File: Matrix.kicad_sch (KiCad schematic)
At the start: 140 parts, among them SW3 RotaryEncoder_Switch

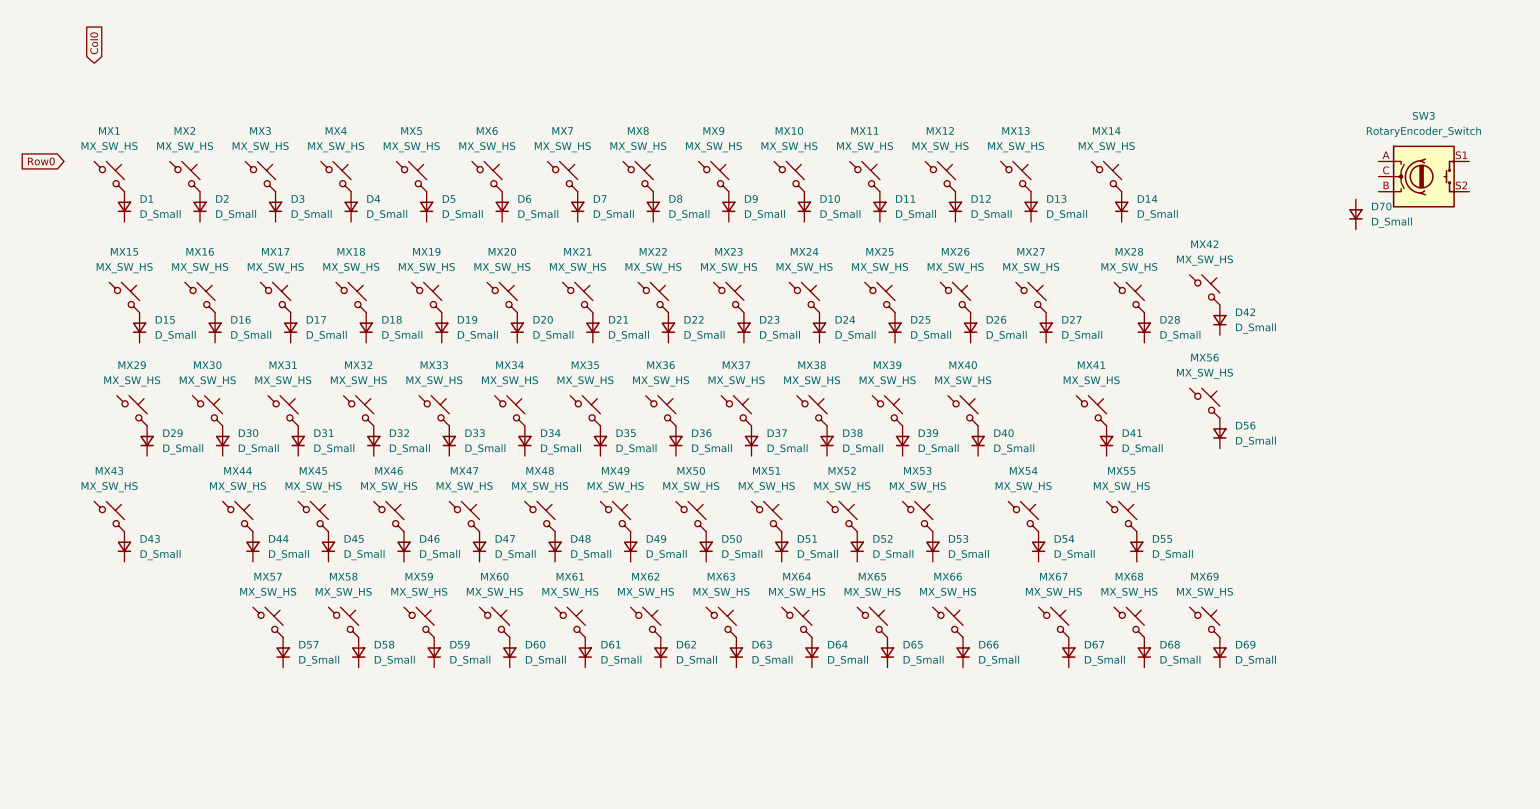
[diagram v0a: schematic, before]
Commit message: Finished switch matrix
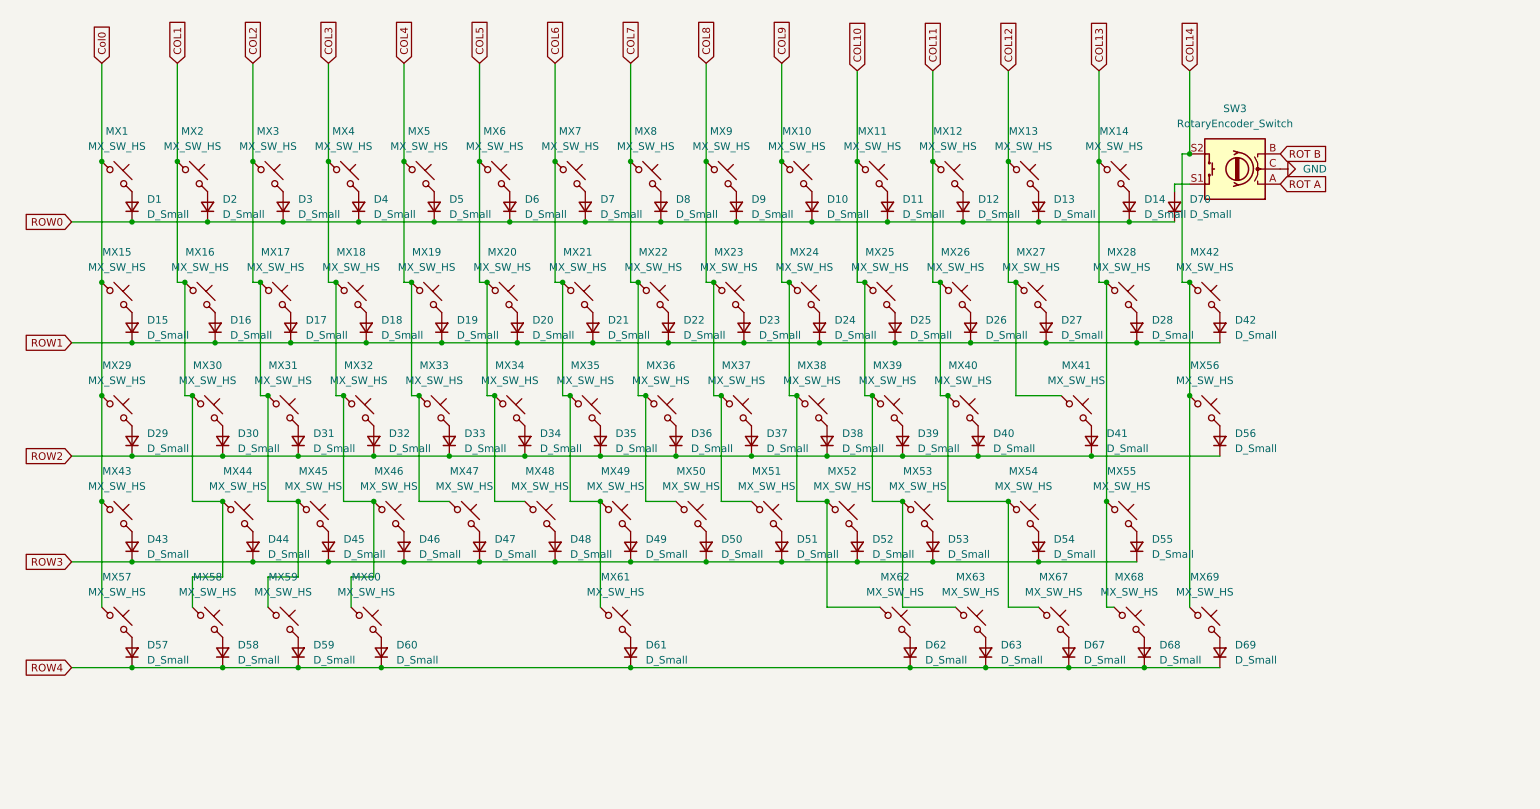
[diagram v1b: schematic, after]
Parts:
- removed D64, D65, D66: D_Small, symbol Device:D_Small
- removed MX64, MX65, MX66: MX_SW_HS, PCM_marbastlib-mx:SW_MX_HS_1u, symbol PCM_marbastlib-mx:MX_SW_HS
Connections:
- net Col0: now also MX1.1, MX15.1, MX29.1, MX43.1, MX57.1
- net COL9: now reaches MX38.1
- net COL9: now also MX10.1, MX24.1, MX52.1, MX62.1
- net COL1: now reaches MX2.1
- net COL1: now also MX16.1, MX30.1, MX44.1, MX58.1
- net COL8: now reaches MX23.1
- net COL8: now also MX37.1, MX51.1, MX9.1
- net COL3: now reaches MX32.1
- net COL3: now also MX18.1, MX4.1, MX46.1, MX60.1
- net COL12: now reaches MX41.1
- net COL12: now also MX13.1, MX27.1
- net COL7: now reaches MX50.1
- net COL7: now also MX22.1, MX36.1, MX8.1
- net COL6: now reaches MX21.1
- net COL6: now also MX35.1, MX49.1, MX61.1, MX7.1
- net ROW2: now reaches D38.1 (K)
- net ROW2: now also D29.1 (K), D30.1 (K), D31.1 (K), D32.1 (K), D33.1 (K), D34.1 (K), D35.1 (K), D36.1 (K), D37.1 (K), D39.1 (K), D40.1 (K), D41.1 (K), D56.1 (K)
- net ROW0: now reaches D70.1 (K)
- net ROW0: now also D1.1 (K), D10.1 (K), D11.1 (K), D12.1 (K), D13.1 (K), D14.1 (K), D2.1 (K), D3.1 (K), D4.1 (K), D5.1 (K), D6.1 (K), D7.1 (K), D8.1 (K), D9.1 (K)
- net at D70.2 (A): now also SW3.S1
- net ROW4: now reaches D62.1 (K)
- net ROW4: now also D57.1 (K), D58.1 (K), D59.1 (K), D60.1 (K), D61.1 (K), D63.1 (K), D67.1 (K), D68.1 (K), D69.1 (K)
- net ROW1: now reaches D23.1 (K)
- net ROW1: now also D15.1 (K), D16.1 (K), D17.1 (K), D18.1 (K), D19.1 (K), D20.1 (K), D21.1 (K), D22.1 (K), D24.1 (K), D25.1 (K), D26.1 (K), D27.1 (K), D28.1 (K), D42.1 (K)
- net COL11: now reaches MX40.1
- net COL11: now also MX12.1, MX26.1, MX54.1, MX67.1
- net COL4: now reaches MX5.1
- net COL4: now also MX19.1, MX33.1, MX47.1
- net ROW3: now reaches D49.1 (K)
- net ROW3: now also D43.1 (K), D44.1 (K), D45.1 (K), D46.1 (K), D47.1 (K), D48.1 (K), D50.1 (K), D51.1 (K), D52.1 (K), D53.1 (K), D54.1 (K), D55.1 (K)
- net COL5: now reaches MX34.1
- net COL5: now also MX20.1, MX48.1, MX6.1
- net COL13: now reaches MX55.1
- net COL13: now also MX14.1, MX28.1, MX68.1
- net COL14: now reaches MX56.1
- net COL14: now also MX42.1, MX69.1, SW3.S2
- net COL2: now reaches MX59.1
- net COL2: now also MX17.1, MX3.1, MX31.1, MX45.1
- net COL10: now reaches MX39.1
- net COL10: now also MX11.1, MX25.1, MX53.1, MX63.1
- net ROT A: now reaches SW3.A
- net ROT B: now reaches SW3.B
- net GND: now reaches SW3.C
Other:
- moved on the sheet: D1, D10, D11, D12, D13, D14, D15, D2, D28, D29, D3, D4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

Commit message: idk
dont remember what i changed lol i think it should be led shit
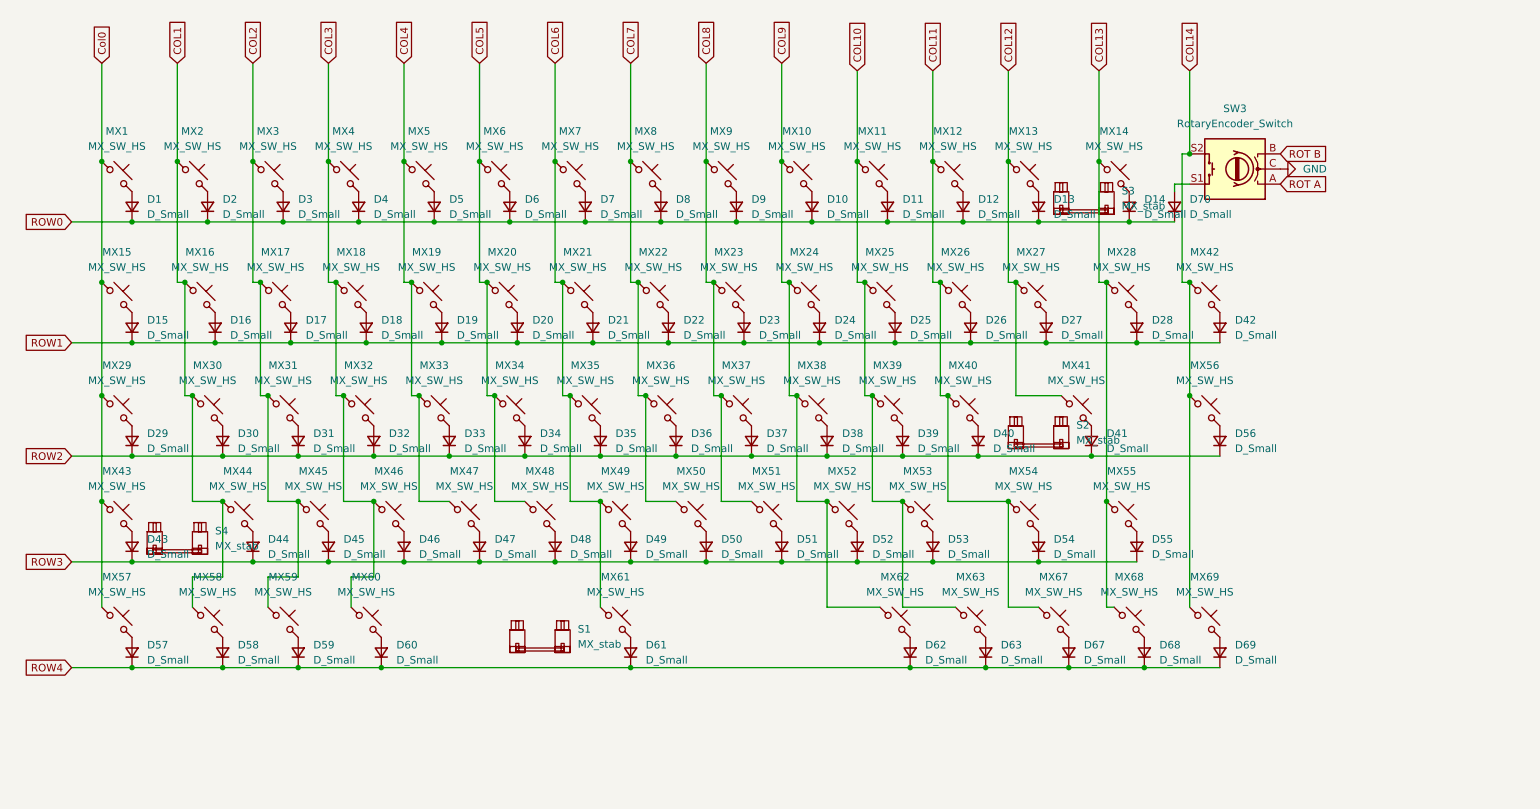
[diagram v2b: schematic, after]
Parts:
- added S1, S2, S3, S4: MX_stab, PCM_marbastlib-mx:STAB_MX_P_6.25u, symbol PCM_marbastlib-mx:MX_stab
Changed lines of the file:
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@@
+    )
+  )
+  (symbol (lib_id "PCM_marbastlib-mx:MX_stab") (at 191.77 55.88 0) (unit 1)
+    (in_bom yes) (on_board yes) (dnp no) (fields_autoplaced)
+    (property "Reference" "S3" (at 198.12 54.483 0)
+      (effects (font (size 1.27 1.27)) (justify left))
+    )
+    (property "Value" "MX_stab" (at 198.12 57.023 0)
+      (effects (font (size 1.27 1.27)) (justify left))
+    )
+    (property "Footprint" "PCM_marbastlib-mx:STAB_MX_P_6.25u" (at 191.77 55.88 0)
+      (effects (font (size 1.27 1.27)) hide)
+    )
+    (property "Datasheet" "" (at 191.77 55.88 0)
+      (effects (font (size 1.27 1.27)) hide)
+    )
+    (instances
+      (project "CODA65"
+        (path "/33ce4dbb-1d04-4b2d-9cde-6cc03c168fa4/fe44eb25-ace8-4884-b9d5-e7eefbf2b910"
+          (reference "S3") (unit 1)
+        )
+      )
     )
   )
@@
     )
   )
+  (symbol (lib_id "PCM_marbastlib-mx:MX_stab") (at 184.15 95.25 0) (unit 1)
+    (in_bom yes) (on_board yes) (dnp no) (fields_autoplaced)
+    (property "Reference" "S2" (at 190.5 93.853 0)
+      (effects (font (size 1.27 1.27)) (justify left))
+    )
+    (property "Value" "MX_stab" (at 190.5 96.393 0)
+      (effects (font (size 1.27 1.27)) (justify left))
+    )
+    (property "Footprint" "PCM_marbastlib-mx:STAB_MX_P_6.25u" (at 184.15 95.25 0)
+      (effects (font (size 1.27 1.27)) hide)
+    )
+    (property "Datasheet" "" (at 184.15 95.25 0)
+      (effects (font (size 1.27 1.27)) hide)
+    )
+    (instances
+      (project "CODA65"
+        (path "/33ce4dbb-1d04-4b2d-9cde-6cc03c168fa4/fe44eb25-ace8-4884-b9d5-e7eefbf2b910"
+          (reference "S2") (unit 1)
+        )
+      )
+    )
+  )
   (symbol (lib_id "PCM_marbastlib-mx:MX_SW_HS") (at 71.12 127 0) (unit 1)
     (in_bom yes) (on_board yes) (dnp no) (fields_autoplaced)
@@
     )
   )
+  (symbol (lib_id "PCM_marbastlib-mx:MX_stab") (at 39.37 113.03 0) (unit 1)
+    (in_bom yes) (on_board yes) (dnp no) (fields_autoplaced)
+    (property "Reference" "S4" (at 45.72 111.633 0)
+      (effects (font (size 1.27 1.27)) (justify left))
+    )
+    (property "Value" "MX_stab" (at 45.72 114.173 0)
+      (effects (font (size 1.27 1.27)) (justify left))
+    )
+    (property "Footprint" "PCM_marbastlib-mx:STAB_MX_P_6.25u" (at 39.37 113.03 0)
+      (effects (font (size 1.27 1.27)) hide)
+    )
+    (property "Datasheet" "" (at 39.37 113.03 0)
+      (effects (font (size 1.27 1.27)) hide)
+    )
+    (instances
+      (project "CODA65"
+        (path "/33ce4dbb-1d04-4b2d-9cde-6cc03c168fa4/fe44eb25-ace8-4884-b9d5-e7eefbf2b910"
+          (reference "S4") (unit 1)
+        )
+      )
+    )
+  )
   (symbol (lib_id "PCM_marbastlib-mx:MX_SW_HS") (at 120.65 91.44 0) (unit 1)
     (in_bom yes) (on_board yes) (dnp no) (fields_autoplaced)
@@
         )
       )
+    )
+  )
+  (symbol (lib_id "PCM_marbastlib-mx:MX_stab") (at 100.33 129.54 0) (unit 1)
+    (in_bom yes) (on_board yes) (dnp no) (fields_autoplaced)
+    (property "Reference" "S1" (at 106.68 128.143 0)
+      (effects (font (size 1.27 1.27)) (justify left))
+    )
+    (property "Value" "MX_stab" (at 106.68 130.683 0)
+      (effects (font (size 1.27 1.27)) (justify left))
+    )
+    (property "Footprint" "PCM_marbastlib-mx:STAB_MX_P_6.25u" (at 100.33 129.54 0)
+      (effects (font (size 1.27 1.27)) hide)
+    )
+    (property "Datasheet" "" (at 100.33 129.54 0)
+      (effects (font (size 1.27 1.27)) hide)
+    )
+    (instances
+      (project "CODA65"
+        (path "/33ce4dbb-1d04-4b2d-9cde-6cc03c168fa4/fe44eb25-ace8-4884-b9d5-e7eefbf2b910"
+          (reference "S1") (unit 1)
+        )
+      )

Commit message: assigned schema
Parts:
- D1, D10, D11, D12, D13, D14, D15, D16, D17, D18, D19, D2, D20, D21, D22, D23, D24, D25, D26, D27, D28, D29, D3, D30, D31, D32, D33, D34, D35, D36, D37, D38, D39, D4, D40, D41, D42, D43, D44, D45, D46, D47, D48, D49, D5, D50, D51, D52, D53, D54, D55, D56, D57, D58, D59, D6, D60, D61, D62, D63, D67, D68, D69, D7, D70, D8, D9: footprint (none) -> Diode_SMD:D_SOD-123
- MX15, MX28: footprint PCM_marbastlib-mx:SW_MX_HS_1u -> PCM_marbastlib-mx:SW_MX_HS_1.5u
- MX29, MX54: footprint PCM_marbastlib-mx:SW_MX_HS_1u -> PCM_marbastlib-mx:SW_MX_HS_1.75u
- MX58, MX63: footprint PCM_marbastlib-mx:SW_MX_HS_1u -> PCM_marbastlib-mx:SW_MX_HS_1.25u
- S2, S4: footprint PCM_marbastlib-mx:STAB_MX_P_6.25u -> PCM_marbastlib-mx:STAB_MX_P_2.25u
- S3: footprint PCM_marbastlib-mx:STAB_MX_P_6.25u -> PCM_marbastlib-mx:STAB_MX_P_2u
- SW3: footprint (none) -> Rotary_Encoder:RotaryEncoder_Alps_EC11E-Switch_Vertical_H20mm

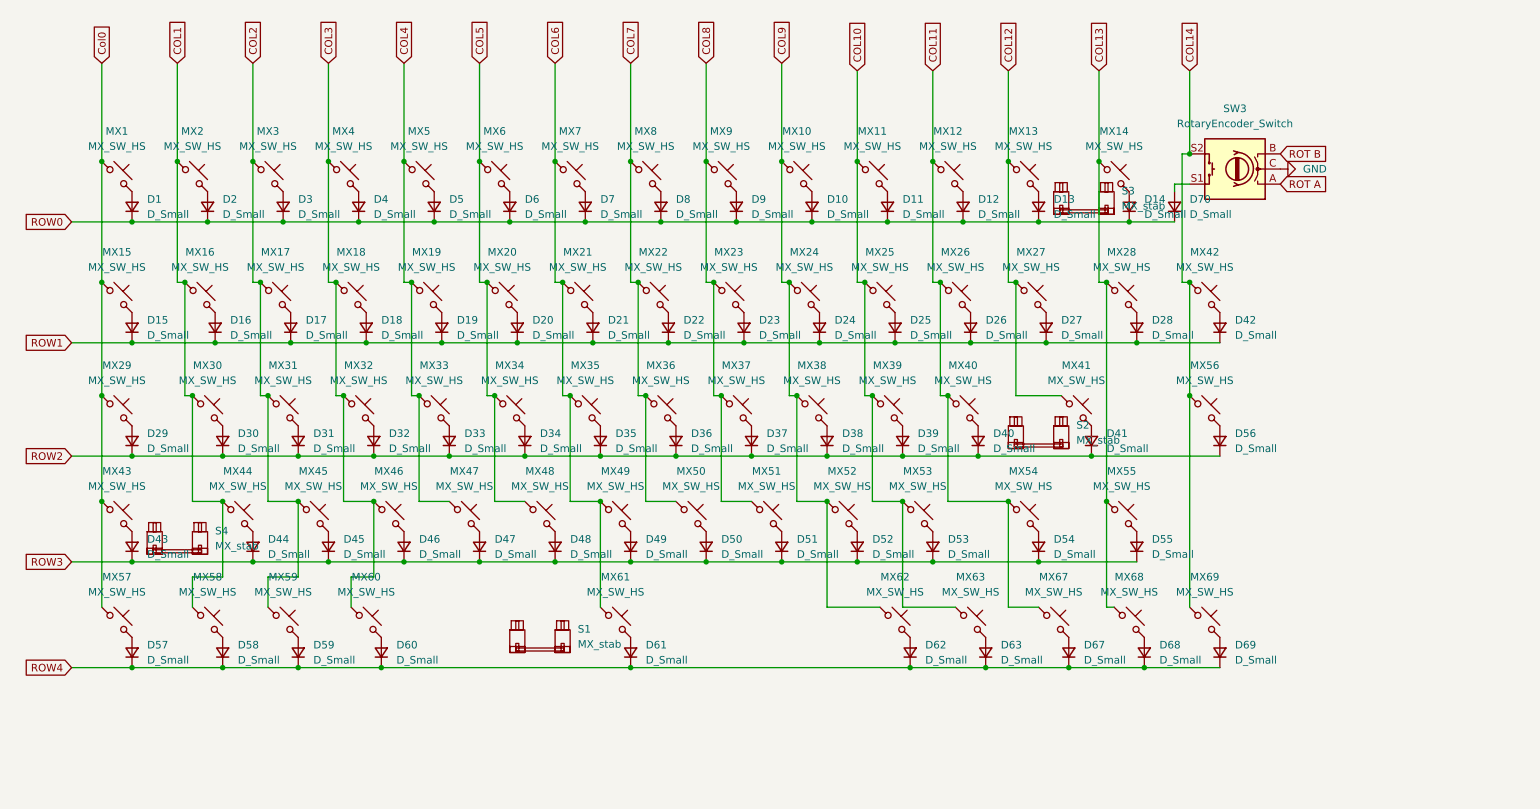
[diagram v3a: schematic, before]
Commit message: Version Update
Moved to latest kicad version
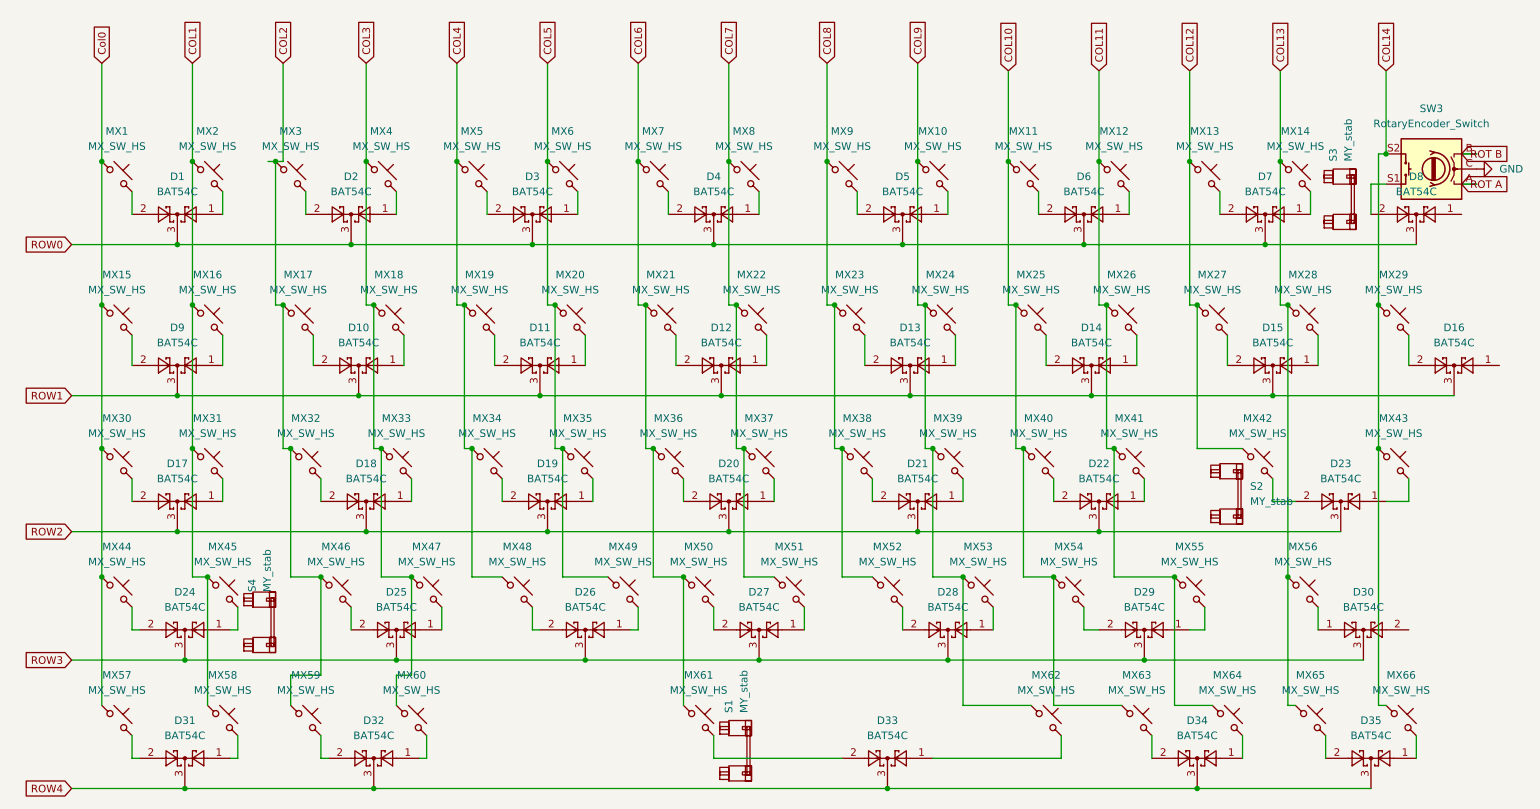
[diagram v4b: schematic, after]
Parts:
- removed D1, D10, D11, D12, D13, D14, D15, D16, D17, D18, D19, D2, D20, D21, D22, D23, D24, D25, D26, D27, D28, D29, D3, D30, D31, D32, D33, D34, D35, D36, D37, D38, D39, D4, D40, D41, D42, D43, D44, D45, D46, D47, D48, D49, D5, D50, D51, D52, D53, D54, D55, D56, D57, D58, D59, D6, D60, D61, D62, D63, D67, D68, D69, D7, D70, D8, D9: D_Small, Diode_SMD:D_SOD-123, symbol Device:D_Small
- added D1, D10, D11, D12, D13, D14, D15, D16, D17, D18, D19, D2, D20, D21, D22, D23, D24, D25, D26, D27, D28, D29, D3, D30, D31, D32, D33, D34, D35, D4, D5, D6, D7, D8, D9: BAT54C, Package_TO_SOT_SMD:SOT-23, symbol Diode:BAT54C
- S1, S2, S3, S4: value MX_stab -> MY_stab
- renumbered MX42 to MX29, MX29 to MX30, MX30 to MX31, MX31 to MX32, MX32 to MX33, MX33 to MX34, MX34 to MX35, MX35 to MX36, MX36 to MX37, MX37 to MX38, MX38 to MX39, MX39 to MX40, MX40 to MX41, MX41 to MX42, MX56 to MX43, MX43 to MX44, MX44 to MX45, MX45 to MX46, MX46 to MX47, MX47 to MX48, MX48 to MX49, MX49 to MX50, MX50 to MX51, MX51 to MX52, MX52 to MX53, MX53 to MX54, MX54 to MX55, MX55 to MX56, MX67 to MX64, MX68 to MX65, MX69 to MX66
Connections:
- net ROW0: now also D1.3, D2.3, D3.3, D4.3, D5.3, D6.3, D7.3, D8.3
- net ROW1: now also D10.3, D11.3, D12.3, D13.3, D14.3, D15.3, D16.3, D9.3
- net ROW2: now also D17.3, D18.3, D19.3, D20.3, D21.3, D22.3, D23.3
- net ROW3: now also D24.3, D25.3, D26.3, D27.3, D28.3, D29.3, D30.3
- net ROW4: now also D31.3, D32.3, D33.3, D34.3, D35.3
- net at MX39.2: now also D21.1
- net at MX2.2: now also D1.1
- net at MX23.2: now also D13.2
- net at MX33.2: now also D18.1
- net at MX42.2: now also D23.2
- net at MX51.2: now also D27.1
- net at MX21.2: now also D12.2
- net at MX31.2: now also D17.1
- net at SW3.S1: now also D8.2
- net at MX61.2: now also D33.2
- net at MX62.2: now also D33.1
- net at MX40.2: now also D22.2
- net at MX36.2: now also D20.2
- net at MX4.2: now also D2.1
- net at MX22.2: now also D12.1
- net at MX41.2: now also D22.1
- net at MX24.2: now also D13.1
- net at MX5.2: now also D3.2
- net at MX25.2: now also D14.2
- net at MX50.2: now also D27.2
- net at MX53.2: now also D28.1
- net at MX60.2: now also D32.1
- net at MX16.2: now also D9.1
- net at MX10.2: now also D5.1
- net at MX7.2: now also D4.2
- net at MX47.2: now also D25.1
- net at MX35.2: now also D19.1
- net at MX8.2: now also D4.1
- net at MX63.2: now also D34.2
- net at MX46.2: now also D25.2
- net at MX56.2: now also D30.1
- net at MX6.2: now also D3.1
- net at MX44.2: now also D24.2
- net at MX65.2: now also D35.2
- net at MX54.2: now also D29.2
- net at MX28.2: now also D15.1
- net at MX20.2: now also D11.1
- net at MX49.2: now also D26.1
- net at MX43.2: now also D23.1
- net at MX59.2: now also D32.2
- net at MX3.2: now also D2.2
- net at MX66.2: now also D35.1
- net at MX57.2: now also D31.2
- net at MX15.2: now also D9.2
- net at MX19.2: now also D11.2
- net at MX26.2: now also D14.1
- net at MX64.2: now also D34.1
- net at MX37.2: now also D20.1
- net at MX30.2: now also D17.2
- net at MX11.2: now also D6.2
- net at MX58.2: now also D31.1
- net at MX1.2: now also D1.2
- net at MX29.2: now also D16.2
- net at MX38.2: now also D21.2
- net at MX9.2: now also D5.2
- net at MX52.2: now also D28.2
- net at MX32.2: now also D18.2
- net at MX27.2: now also D15.2
- net at MX13.2: now also D7.2
- net at MX18.2: now also D10.1
- net at MX55.2: now also D29.1
- net at MX14.2: now also D7.1
- net at MX12.2: now also D6.1
- net at MX17.2: now also D10.2
- net at MX34.2: now also D19.2
- net at MX48.2: now also D26.2
- net at MX45.2: now also D24.1
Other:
- moved on the sheet: MX10, MX11, MX12, MX13, MX14, MX15, MX16, MX17, MX18, MX19, MX2, MX20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
